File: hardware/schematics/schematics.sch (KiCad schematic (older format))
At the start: 22 parts, among them J1 Jack-DC, Q1 Q_NMOS_DGS, U1 L7805, U2 ESP32-DevKitC, U3 MAX6921AUI+

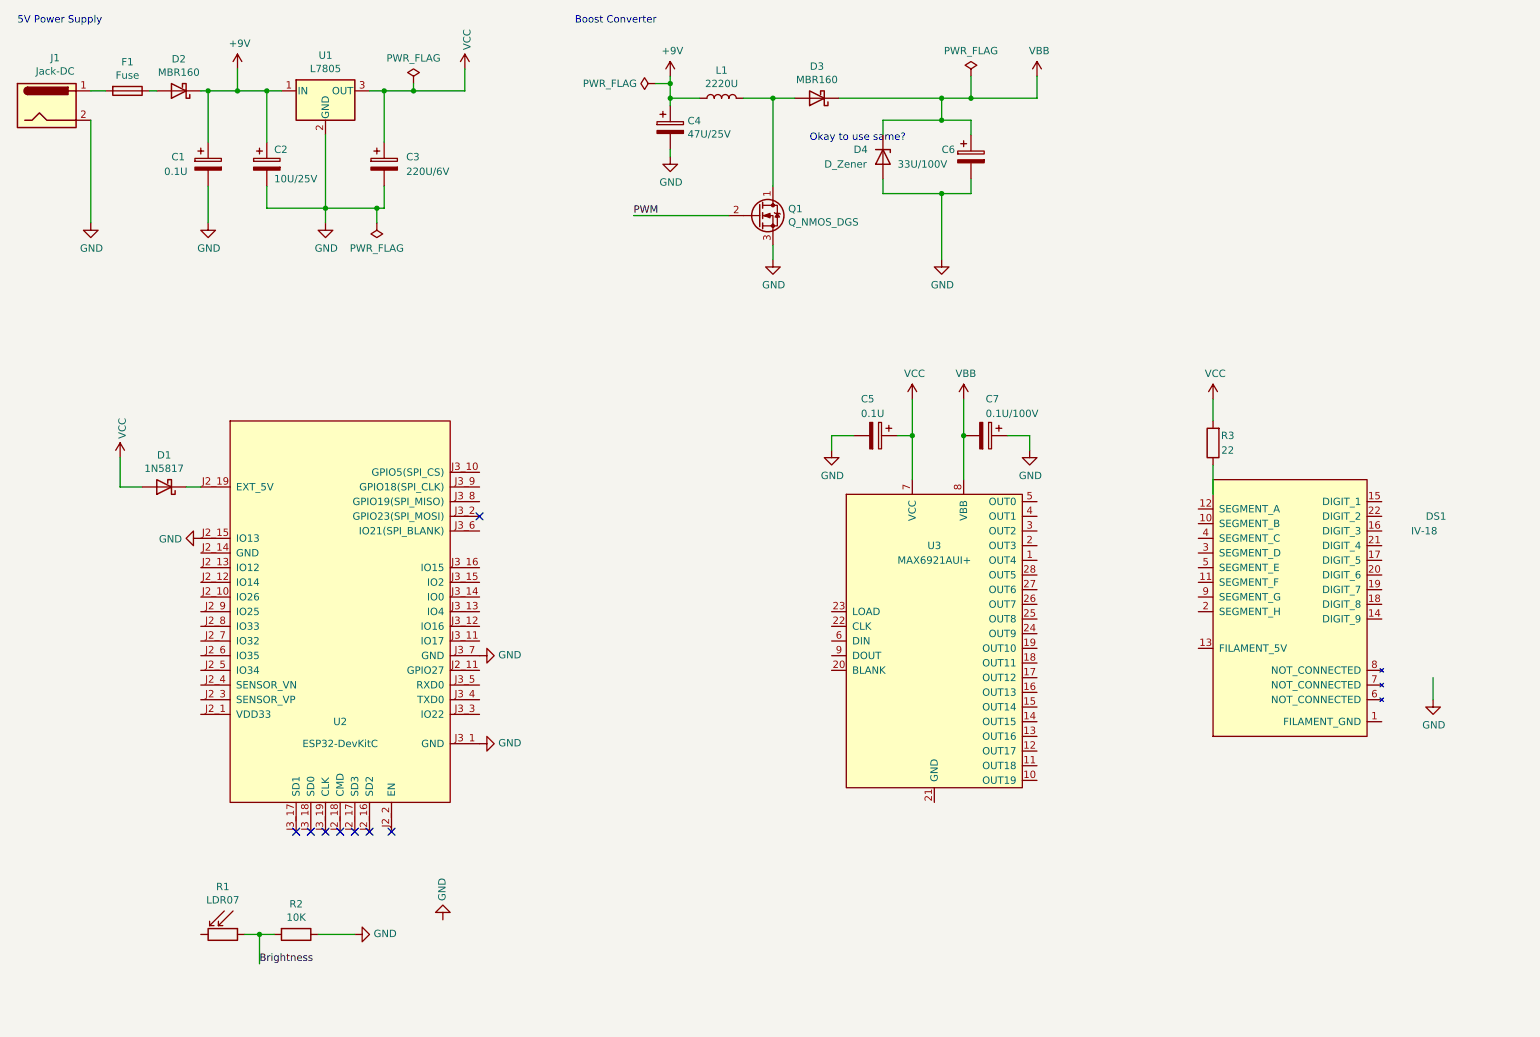
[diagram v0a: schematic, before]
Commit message: Schematics completed
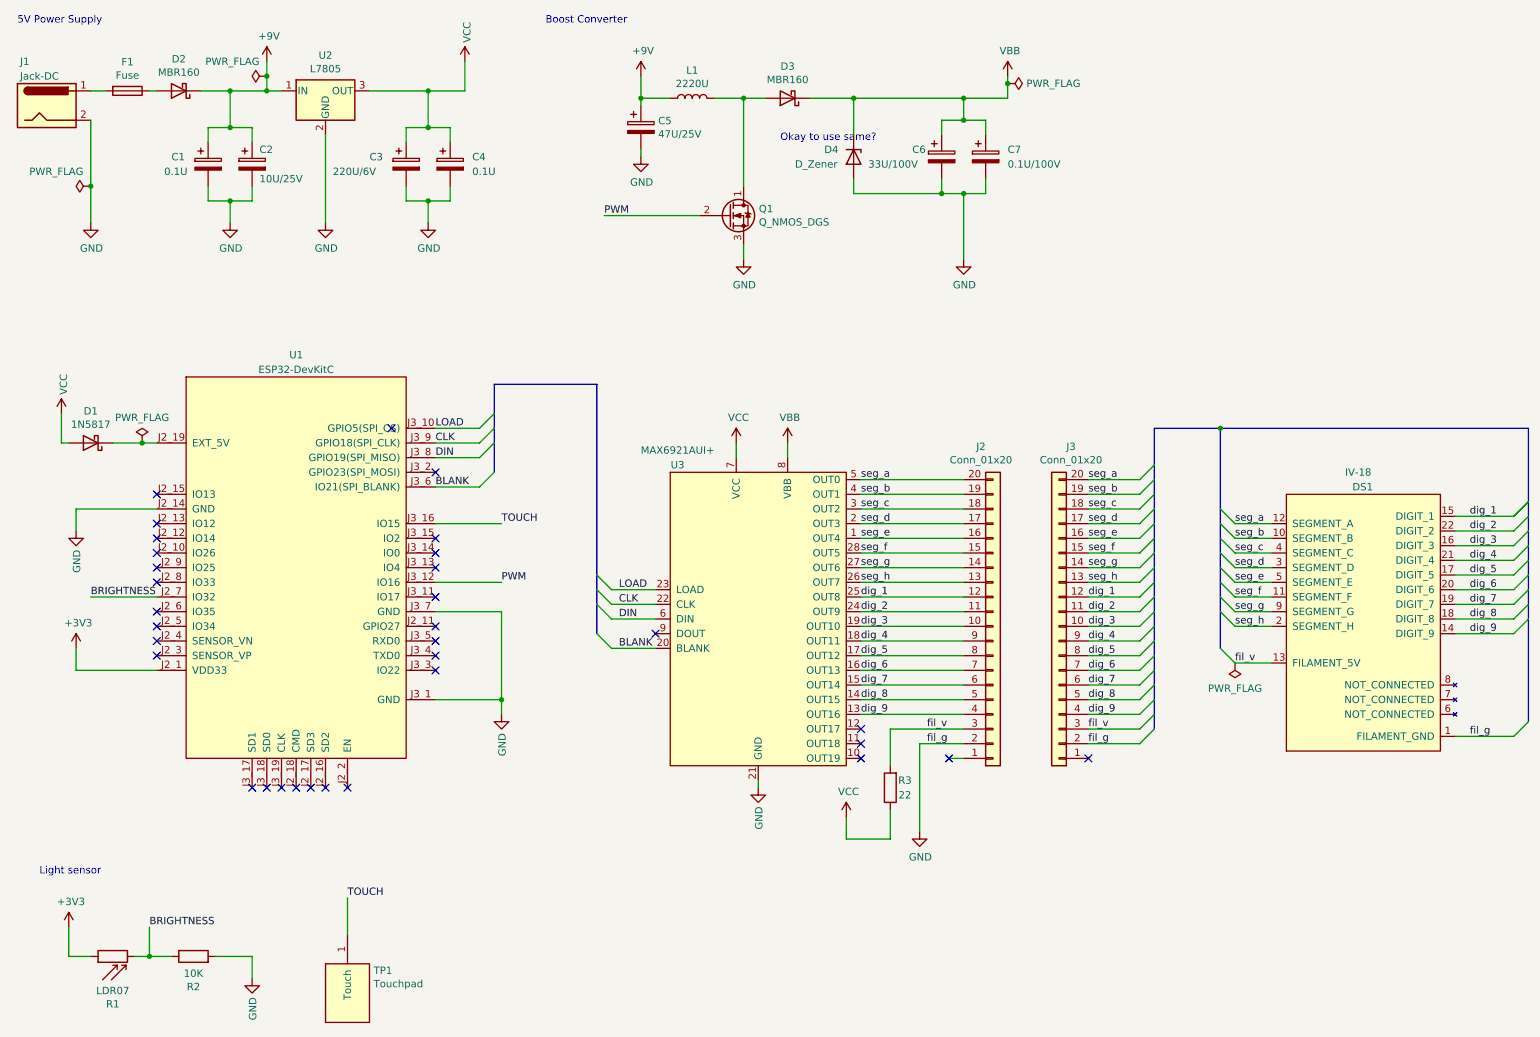
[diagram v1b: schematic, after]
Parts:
- added J2, J3: Conn_01x20, Connector_PinHeader_2.54mm:PinHeader_2x10_P2.54mm_Vertical, symbol Connector_Generic:Conn_01x20
- added TP1: Touchpad, Connector_PinSocket_2.54mm:PinSocket_1x01_P2.54mm_Vertical, symbol callisto_lib:Touchpad
- DS1: footprint Connector_PinHeader_1.27mm:PinHeader_2x10_P1.27mm_Vertical -> callisto:IV-18
- renumbered C5 to C4, C4 to C5, U2 to U1, U1 to U2
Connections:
- net labels added: +3V3, BLANK, BRIGHTNESS, CLK, DIN, LOAD, TOUCH, dig_1, dig_2, dig_3, dig_4, dig_5, dig_6, dig_7, dig_8, dig_9, fil_g, fil_v, seg_a, seg_b, seg_c, seg_d, seg_e, seg_f, seg_g, seg_h
- net labels removed: Brightness
- wire segments 70 -> 157
- no-connect marks 8 -> 33
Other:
- note added: "Light sensor"
- moved on the sheet: C2, C3, C4, C5, C6, C7, D1, D3, D4, DS1, L1, Q1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
